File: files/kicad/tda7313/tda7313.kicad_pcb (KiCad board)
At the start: 2 copper layers, 62.2 x 59.7 mm, 36 parts, among them J1 SP_L, J10 OUT_FL, J11 OUT_RL, J12 OUT_FR, J13 OUT_RR, J14 PWR, J2 IN1_L, J3 IN2_L, J4 IN3_L, J5 IN1_R, J6 IN2_R, J7 IN3_R, J8 SP_R, J9 I2C, U1 TDA7313

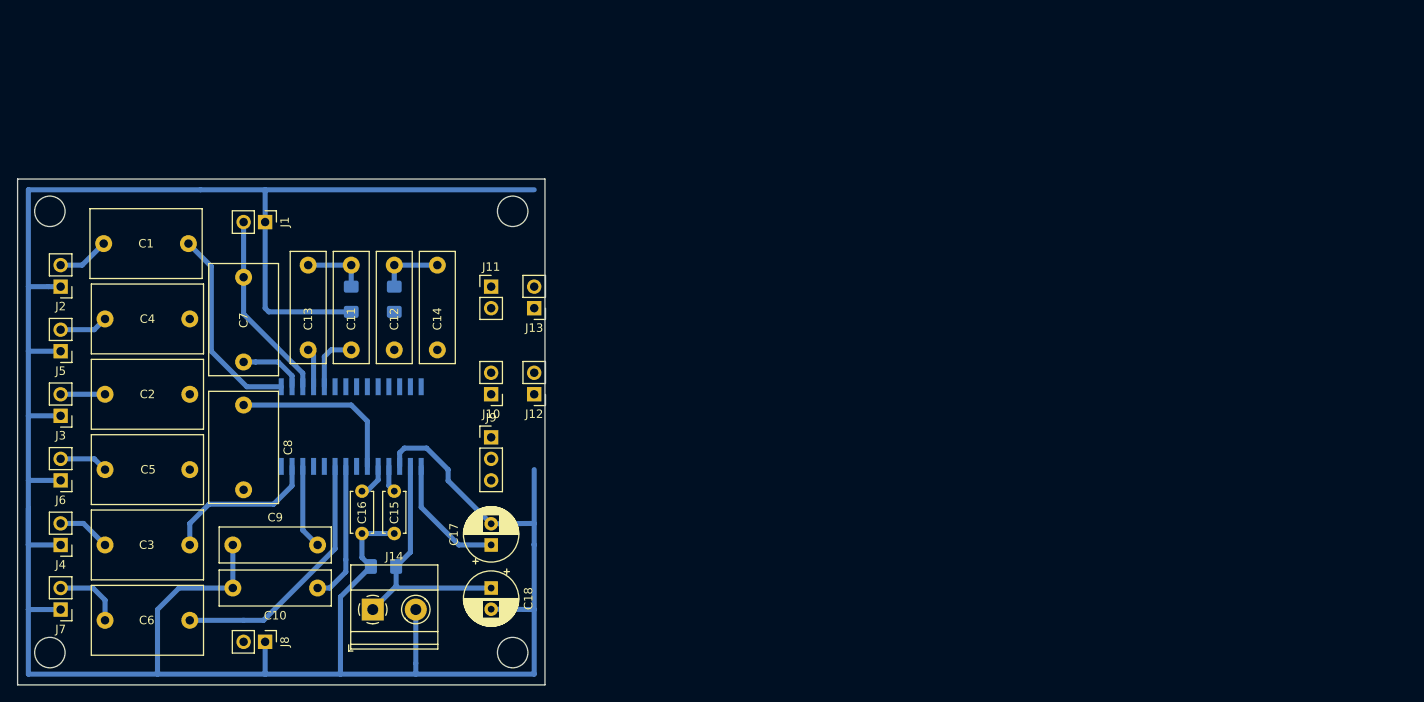
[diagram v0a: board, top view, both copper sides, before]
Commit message: PCB for TDA7313
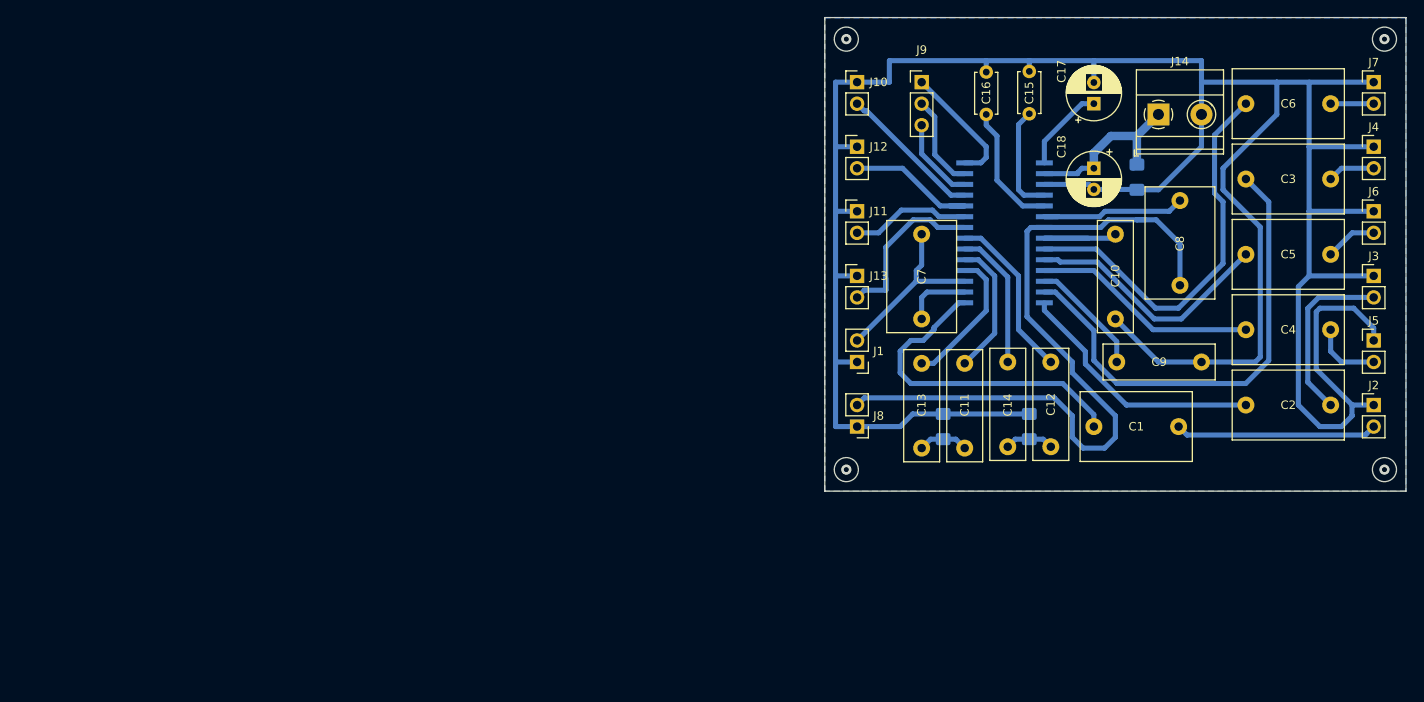
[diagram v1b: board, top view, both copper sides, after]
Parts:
- moved J7 167.0 mm to (251.5, 68.6), turned to 0 degrees
- moved J4 161.9 mm to (251.5, 76.2), turned to 0 degrees
- moved J6 158.2 mm to (251.5, 83.8), turned to 0 degrees
- moved J3 155.8 mm to (251.5, 91.4), turned to 0 degrees
- moved J2 155.6 mm to (251.5, 106.7), turned to 0 degrees
- moved J5 154.9 mm to (251.5, 99.1), turned to 0 degrees
- moved C6 138.7 mm to (236.4, 71.1), turned to 0 degrees
- moved C3 131.9 mm to (236.4, 80.0), turned to 0 degrees
- moved C5 127.2 mm to (236.4, 88.9), turned to 0 degrees
- moved C2 124.6 mm to (236.4, 106.7), turned to 0 degrees
- moved C4 124.6 mm to (236.4, 97.8), turned to 0 degrees
- moved C9 116.3 mm to (231.1, 101.6), turned to 180 degrees
- moved C8 113.1 mm to (228.6, 82.5)
- moved J14 109.6 mm to (226.1, 72.4)
- moved C1 109.0 mm to (218.4, 109.2), turned to 0 degrees
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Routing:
- net Net-(C8-Pad2): track 0.00 -> 89.6 mm
- net Net-(C3-Pad1): track 18.7 -> 56.7 mm
- net Net-(C2-Pad1): track 0.00 -> 30.2 mm
- net Net-(C5-Pad1): track 0.00 -> 29.8 mm
- net Net-(C4-Pad1): track 0.00 -> 28.3 mm
- net Net-(J13-Pad2): track 0.00 -> 21.3 mm
- net Net-(C12-Pad1): track 0.00 -> 19.9 mm
- net Net-(C1-Pad2): track 6.13 -> 23.8 mm
- net Net-(J10-Pad2): track 0.00 -> 17.2 mm
- net Net-(C6-Pad1): track 30.4 -> 47.0 mm
- net Net-(C14-Pad1): track 0.00 -> 16.5 mm
- net Net-(J12-Pad2): track 0.00 -> 16.3 mm
- net Net-(C2-Pad2): track 5.24 -> 20.8 mm
- net Net-(C1-Pad1): track 23.8 -> 39.0 mm
- net Net-(J9-Pad1): track 0.00 -> 14.8 mm
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- added copper zone on B.Cu, net GNDA
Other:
- board size 62.2 x 59.7 mm -> 68.6 x 55.9 mm
